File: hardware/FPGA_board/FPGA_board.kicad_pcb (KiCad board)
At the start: 6 copper layers, 50.9 x 24.8 mm, 142 parts, among them J1 USB_C_Receptacle_USB2.0, J2 Conn_01x6_Male, J3 USB_C_Receptacle_USB2.0, J4 MicroSd, J5 Conn_01x03, J6 JTAG, J7 Conn_02x15_Odd_Even, J8 Conn_02x15_Odd_Even, SW1 SW_Push, U1 RY1303 or EA3036, U10 NCP115-2.5, U3 ECP5U25, U4 MT41K64M16TW-107_J-TR, U6 XT25Q08DDTIGT, U8 TPS51206

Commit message: update PCB design files
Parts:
- added G***: LOGO, LOGO, B.Cu at (176.1, 92.9)
- added G***: LOGO, LOGO, B.Cu at (162.9, 93.3)

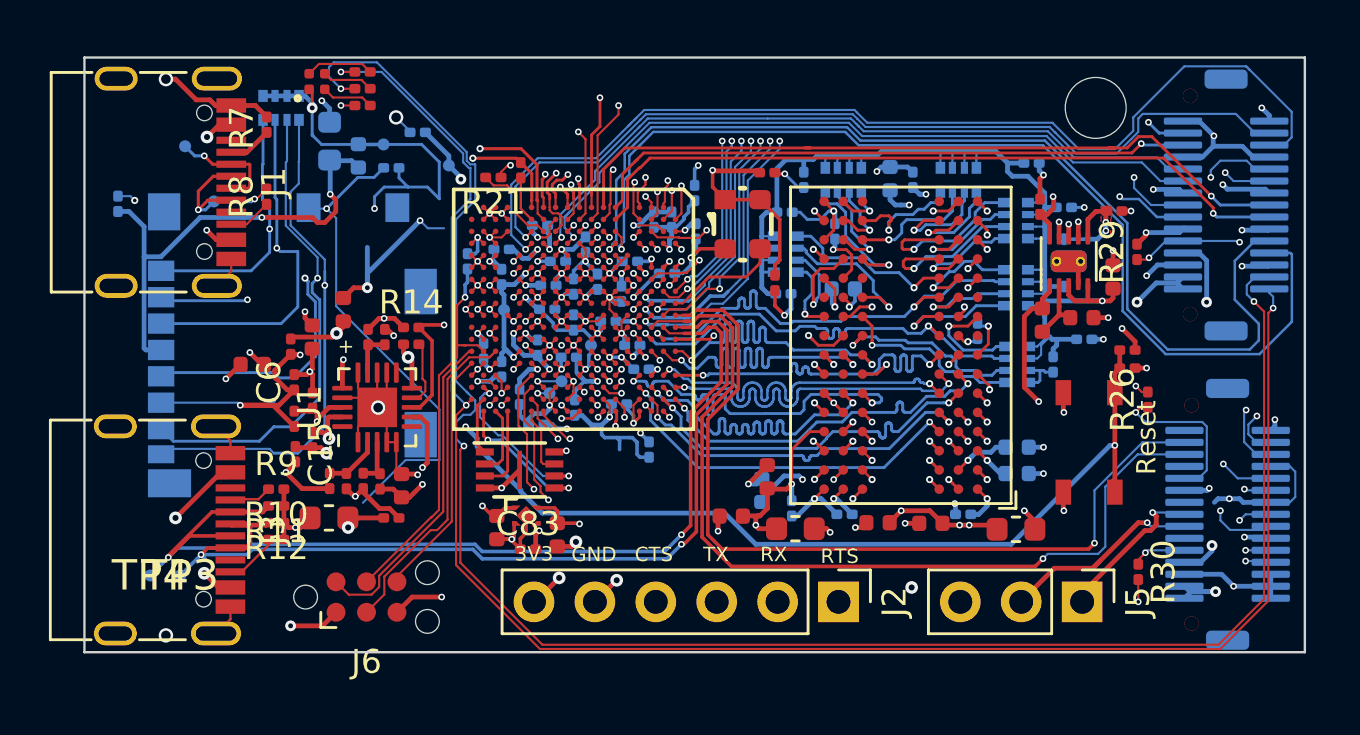
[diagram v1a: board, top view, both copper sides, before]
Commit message: update PCB design files
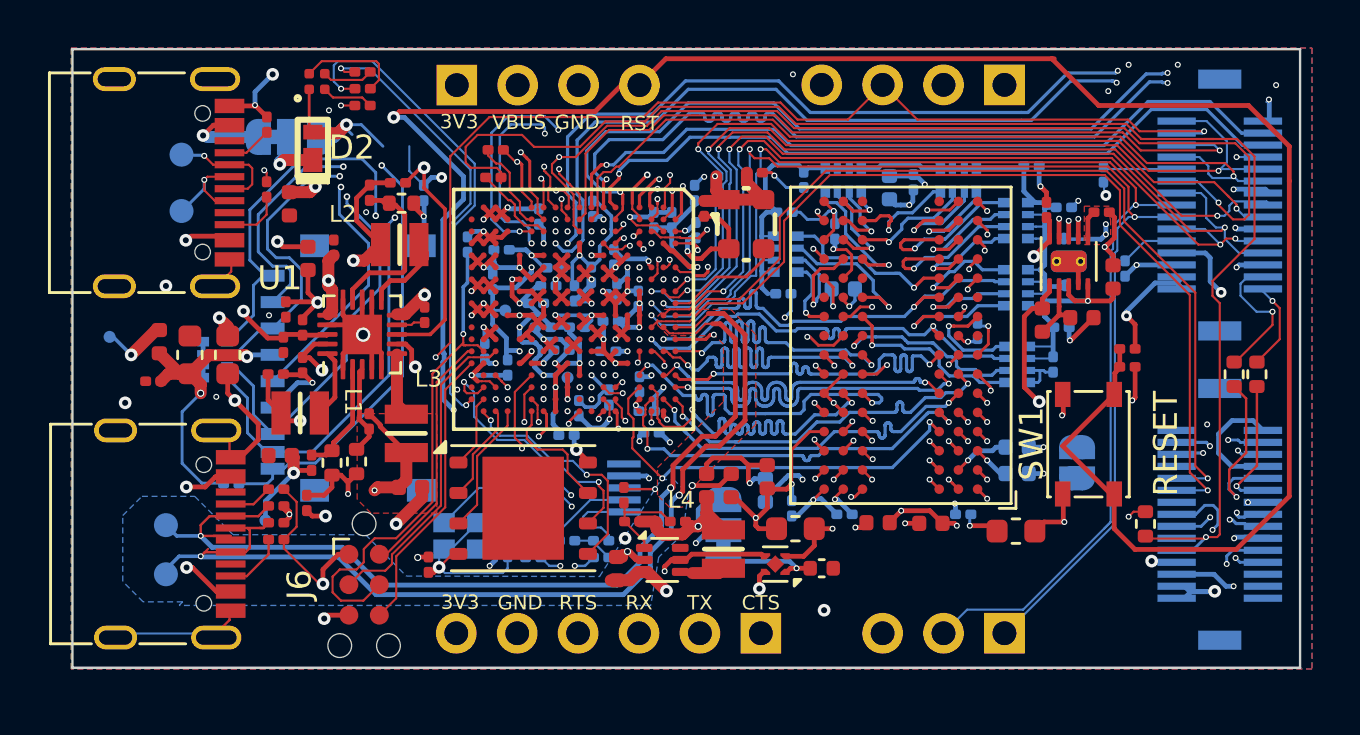
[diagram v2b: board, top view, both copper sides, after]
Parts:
- removed the G*** at (176.1, 92.9)
- removed the G*** at (162.9, 93.3)
- removed H4: MountingHole, MountingHole:MountingHole_2.1mm
- removed J1, J3: USB_C_Receptacle_USB2.0, Connector_USB:USB_C_Receptacle_G-Switch_GT-USB-7010ASV
- removed TP19, TP20: SMD_TP, gkl_misc:TestPoint_Pad_D0.5mm
- removed TP3, TP4: , 
- removed U10: NCP115-2.5, gkl_housings_son:X2SON_4_1.0x1.0mm
- added C13: 100pF, Capacitor_SMD:C_0201_0603Metric, F.Cu at (164.8, 109.8)
- added C28: 4.7uF, Capacitor_SMD:C_0402_1005Metric, F.Cu at (170.8, 111.7)
- added C29: 100nF, Capacitor_SMD:C_0201_0603Metric, B.Cu at (157.7, 110.9)
- added D2: D_Schottky, Library:U-DFN1608-2_L1.6-W0.8-RD, F.Cu at (149.5, 94.1)
- added G***: LOGO, LOGO, B.Cu at (171.0, 104.0)
- added G***: LOGO, LOGO, B.Cu at (182.6, 109.8)
- added J10: Conn_01x04, Connector_PinHeader_2.54mm:PinHeader_1x04_P2.54mm_Vertical, B.Cu at (155.5, 91.5)
- added J9: TF TF-018 1.5mm, Library:TF-SMD_TF-018, B.Cu at (149.7, 103.6)
- added JP1: SolderJumper_3_Bridged12, Jumper:SolderJumper-3_P1.3mm_Bridged12_RoundedPad1.0x1.5mm, B.Cu at (148.5, 93.7)
- added JP2: SolderJumper_3_Bridged12, Jumper:SolderJumper-3_P1.3mm_Bridged12_RoundedPad1.0x1.5mm, B.Cu at (166.7, 110.1)
- added JP3: SolderJumper_2_Open, Jumper:SolderJumper-2_P1.3mm_Open_RoundedPad1.0x1.5mm, B.Cu at (181.4, 107.3)
- added L1: 2.2uH, Library:Murata_DFE201612P-2R2M=P2, F.Cu at (149.0, 105.2)
- added L2: 2.2uH, Library:Murata_DFE201612P-2R2M=P2, F.Cu at (153.2, 98.2)
- added L3: 2.2uH, Library:Murata_DFE201612P-2R2M=P2, F.Cu at (153.4, 106.1)
- added L4: 2.2uH, Library:Murata_DFE201612P-2R2M=P2, F.Cu at (166.7, 110.9)
- added R31: 22, Resistor_SMD:R_0402_1005Metric, F.Cu at (188.9, 103.6)
- added R32: 22, Resistor_SMD:R_0402_1005Metric, F.Cu at (187.9, 103.6)
- added R33: 15k, Resistor_SMD:R_0201_0603Metric, F.Cu at (162.8, 109.8)
- added R34: 4.7k, Resistor_SMD:R_0201_0603Metric, F.Cu at (162.5, 108.7)
- added R35: 15, Resistor_SMD:R_0201_0603Metric, B.Cu at (161.6, 110.5)
- added R36: 15, Resistor_SMD:R_0201_0603Metric, B.Cu at (158.7, 110.5)
- added R37: 75, Resistor_SMD:R_0201_0603Metric, B.Cu at (160.1, 110.5)
- added R38: 15, Resistor_SMD:R_0201_0603Metric, B.Cu at (161.6, 111.2)
- added R39: 15, Resistor_SMD:R_0201_0603Metric, B.Cu at (158.7, 111.2)
- added TP1: SMD_TP, TestPoint:TestPoint_Pad_D1.0mm, B.Cu at (143.4, 112.0)
- added TP2: SMD_TP, TestPoint:TestPoint_Pad_D1.0mm, B.Cu at (143.4, 109.9)
- added U2: TLV62569APDRL, Package_TO_SOT_SMD:SOT-563, F.Cu at (164.1, 111.3)
- added U5: Si5351A-B-GT, Package_SO:MSOP-10_3x3mm_P0.5mm, B.Cu at (160.3, 108.3)
- added U7: NCP115AMX250TCG, Package_DFN_QFN:OnSemi_XDFN4-1EP_1.0x1.0mm_EP0.52x0.52mm, F.Cu at (168.8, 111.5)
- added USBD1: USB_C_Receptacle_USB2.0, Connector_USB:USB_C_Receptacle_G-Switch_GT-USB-7010ASV, F.Cu at (142.3, 95.6)
- added USBH1: USB_C_Receptacle_USB2.0, Connector_USB:USB_C_Receptacle_G-Switch_GT-USB-7010ASV, F.Cu at (142.4, 110.3)
- added Y1: 27MHz, Crystal:Crystal_SMD_2016-4Pin_2.0x1.6mm, B.Cu at (155.7, 110.3)
- C70, C71, FB1: moved to F.Cu
- J2, J5, R26, R30: moved to B.Cu
- J4: value MicroSd -> Conn_01x04_Male; footprint Connector_Card:microSD_HC_Molex_104031-0811 -> Connector_PinHeader_2.54mm:PinHeader_1x04_P2.54mm_Vertical
- J7, J8: footprint gkl_conn:DF12(3.0)-30DP-0.5V(86) -> Library:DF12NB3030DP05V51
- R10, R9: value 51K -> 12K
- R15: value 120K -> 120K 1%; footprint Resistor_SMD:R_0201_0603Metric -> Resistor_SMD:R_0402_1005Metric
- R16: value 82K -> 82K 1%; footprint Resistor_SMD:R_0201_0603Metric -> Resistor_SMD:R_0402_1005Metric
- R17, R18, R5: value 100k -> 100k 1%
- R2: value 22K -> 22K 1%; footprint Resistor_SMD:R_0201_0603Metric -> Resistor_SMD:R_0402_1005Metric
- R29: footprint Resistor_SMD:R_0201_0603Metric -> Resistor_SMD:R_0402_1005Metric
- SW1: footprint gkl_misc:PTS_810_SMT_Switch -> Button_Switch_SMD:SW_SPST_PTS810
- TP26, TP27: footprint gkl_misc:TestPoint_Pad_D0.5mm -> TestPoint:TestPoint_Pad_D1.0mm
- TP28, TP29, TP30, TP31, TP32, TP33: footprint gkl_misc:TestPoint_Pad_D0.5mm -> Library:TestPoint_Pad_D0.5mm
- U3: value ECP5U25 -> ECP5
- U6: value XT25Q08DDTIGT -> W25Q128JVPIQ; footprint gkl_housings_dfn:DFN-8-1EP_3x2mm_Pitch0.5mm -> Package_SON:WSON-8-1EP_6x5mm_P1.27mm_EP3.4x4.3mm
- moved J4 31.6 mm to (178.4, 91.5), turned to 90 degrees
- moved TP32 15.4 mm to (147.6, 109.7), turned to 180 degrees
- moved R28 14.8 mm to (146.1, 108.2), turned to 0 degrees
- moved TP29 14.0 mm to (141.1, 102.0), turned to 180 degrees
- moved R30 12.7 mm to (183.4, 99.2)
- moved FB1 11.4 mm to (143.1, 102.2)
- moved R29 11.4 mm to (184.2, 109.8)
- moved RN7 10.9 mm to (145.4, 103.0), turned to 180 degrees
- moved C71 10.6 mm to (144.4, 102.8)
- moved TP31 10.1 mm to (160.2, 103.8), turned to 180 degrees
- moved R26 9.58 mm to (182.5, 95.3), turned to -90 degrees
- moved C47 8.93 mm to (165.9, 108.2), turned to 90 degrees
- moved C3 8.01 mm to (146.0, 102.8), turned to 90 degrees
- moved C70 7.55 mm to (142.9, 103.9), turned to 0 degrees
- moved R14 6.06 mm to (153.1, 95.6)
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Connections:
- net USB_PULLUP renamed PULLUP_USB
- C11 pad 1: GND -> VTT
- C11 pad 2: VTT -> GND
- C14 pad 2: PUSB_VBUS -> VSYS
- C17 pad 1: GND -> P1.1V
- C17 pad 2: P1.1V -> GND
- C18 pad 1: GND -> P1.35V
- C18 pad 2: P1.35V -> GND
- C2 pad 2: PUSB_VBUS -> VSYS
- C3 pad 2: PUSB_VBUS -> VSYS
- C47 pad 1: P2.5V -> Net-(JP2-B)
- C5 pad 2: PUSB_VBUS -> VSYS
- C7 pad 1: GND -> P3.3V
- C7 pad 2: P3.3V -> GND
- C70 pad 2: Net-(J4-Pin_4) -> /sheetSDMMC/VDD_SD
- C71 pad 1: Net-(J4-Pin_4) -> /sheetSDMMC/VDD_SD
- FB1 pad 1: Net-(J4-Pin_4) -> /sheetSDMMC/VDD_SD
- J2 pad 1: IO_1 -> IO_MISO
- J2 pad 2: IO_0 -> IO_1
- J2 pad 3: IO_MISO -> IO_0
- J4 pad 1: SD0_DAT2 -> IO_10
- J4 pad 2: SD0_DAT3 -> IO_9
- J4 pad 3: SD0_CMD -> IO_SCK
- J4 pad 4: Net-(J4-Pin_4) -> IO_13
- J5 pad 1: IO_SDA -> IO_SCL
- J5 pad 2: IO_SCL -> IO_SDA
- J7 pad 1: GND -> IO_11
- J7 pad 10: AUX_1- -> IO_11
- J7 pad 11: AUX_4+ -> LED_B
- J7 pad 12: AUX_1+ -> IO_12
- J7 pad 13: GND -> IO_6
- J7 pad 15: AUX_5- -> IO_SDA
- J7 pad 16: AUX_2- -> IO_9
- J7 pad 17: AUX_5+ -> IO_SCL
- J7 pad 18: AUX_2+ -> IO_10
- J7 pad 19: GND -> IO_5
- J7 pad 21: HPD/ID -> Net-(J7-Pin_21)
- J7 pad 22: AUX_6+ -> IO_5
- J7 pad 24: AUX_6- -> IO_6
- J7 pad 28: LED_G -> Net-(J7-Pin_28)
- J7 pad 3: AUX_3- -> IO_SCK
- J7 pad 30: LED_R -> Net-(J7-Pin_30)
- J7 pad 4: AUX_0- -> AUX_3-
- J7 pad 5: AUX_3+ -> IO_13
- J7 pad 6: AUX_0+ -> AUX_3+
- J7 pad 7: GND -> IO_12
- J7 pad 9: AUX_4- -> Net-(J7-Pin_9)
- J7 pad MP: (no net) -> GND
- J8 pad 10: IO_11 -> AUX_1-
- J8 pad 11: LED_B -> SPI_1
- J8 pad 12: IO_12 -> AUX_1+
- J8 pad 15: IO_SDA -> AUX_5-
- J8 pad 16: IO_9 -> AUX_2-
- J8 pad 17: IO_SCL -> AUX_5+
- J8 pad 18: IO_10 -> AUX_2+
- J8 pad 21: Net-(J8-Pin_21) -> HPD/ID
- J8 pad 22: IO_5 -> AUX_6+
- J8 pad 24: IO_6 -> AUX_6-
- J8 pad 3: SPI_0 -> AUX_4-
- J8 pad 4: IO_SCK -> AUX_0-
- J8 pad 5: SPI_1 -> AUX_4+
- J8 pad 6: IO_13 -> AUX_0+
- J8 pad 9: Net-(J8-Pin_9) -> SPI_0
- J8 pad MP: (no net) -> GND
- R10 pad 1: Net-(J3-CC2) -> P3.3V
- R10 pad 2: GND -> Net-(USBH1-CC2)
- R22 pad 1: LED_R -> LED_G
- R23 pad 1: LED_G -> LED_R
- R26 pad 1: Net-(J8-Pin_9) -> Net-(J7-Pin_9)
- R28 pad 1: P3.3V -> /sheetSDMMC/VDD_SD
- R30 pad 1: Net-(J8-Pin_21) -> Net-(J7-Pin_21)
- R9 pad 1: Net-(J3-CC1) -> P3.3V
- R9 pad 2: GND -> Net-(USBH1-CC1)
- RN7 pad 1: SD0_DAT1 -> SD0_DAT2
- RN7 pad 2: SD0_DAT0 -> SD0_CMD
- RN7 pad 3: SD0_CMD -> SD0_DAT0
- RN7 pad 4: SD0_DAT2 -> SD0_DAT1
- RN7 pad 5: P3.3V -> /sheetSDMMC/VDD_SD
- RN7 pad 6: P3.3V -> /sheetSDMMC/VDD_SD
- RN7 pad 7: P3.3V -> /sheetSDMMC/VDD_SD
- RN7 pad 8: P3.3V -> /sheetSDMMC/VDD_SD
- U1 pad 16: PUSB_VBUS -> VSYS
- U1 pad 19: PUSB_VBUS -> VSYS
- U1 pad 7: PUSB_VBUS -> VSYS
- U4 pad G8: (no net) -> GND
- U4 pad J1: (no net) -> unconnected-(U4-PadJ1)
- U4 pad J9: (no net) -> unconnected-(U4-PadJ9)
- U4 pad L1: (no net) -> unconnected-(U4-PadL1)
- U4 pad L9: (no net) -> unconnected-(U4-PadL9)
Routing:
- net P3.3V: track 174.3 -> 241.5 mm, vias 22 -> 21
- net LED_G: track 80.7 -> 22.8 mm, vias 4 -> 3
- net LED_R: track 74.8 -> 18.7 mm, vias 3 -> 2
- net FPGA_RESET: track 41.1 -> 90.9 mm
- net VSYS: track 0.00 -> 44.7 mm, vias 0 -> 6
- net /sheetHyperRAM/RAM_VDD: track 18.1 -> 60.0 mm, vias 12 -> 11
- net IO_SDA: track 44.1 -> 73.9 mm, vias 3 -> 4
- net AUX_2+: track 30.2 -> 57.3 mm, vias 1 -> 3
- net IO_SCL: track 47.5 -> 73.6 mm, vias 3 -> 4
- net AUX_4+: track 30.6 -> 55.5 mm, vias 1 -> 3
- net AUX_4-: track 30.1 -> 54.9 mm, vias 1 -> 3
- net AUX_2-: track 31.7 -> 55.4 mm, vias 1 -> 3
- net /sheetPower/PGOOD_P1.1V: track 16.5 -> 38.3 mm, vias 2 -> 3
- net /sheetHyperRAM/RAM_VDDQ: track 15.6 -> 36.4 mm
- net AUX_1-: track 34.4 -> 54.9 mm
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- added copper zone on In2.Cu, net (none)
- added copper zone on B.Cu, net GND
- added copper zone on F.Cu, net GND
- added copper zone on F.Cu, net P1.35V
- added copper zone on In1.Cu, net P1.35V
- added copper zone on In2.Cu, net P2.5V
- added copper zone on In2.Cu, net P3.3V
- added copper zone on In1.Cu, net PUSB_VBUS
- added copper zone on In3.Cu, net VSYS
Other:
- board size 50.9 x 24.8 mm -> 51.2 x 25.8 mm
- board text added: "0.275/.15 via handles 1.6A .53/.25 via handles 2.2A .5 track (external) handles 1.4A .2 track (external) handles .73A internal tracks: 5x"
- board text added: "90ohm JLC06161H-3313A coplanar -trace spacing/clearance: .2032mm width: .1554mm"
- board text added: "Avaota-A1 design BGA pad: 0.2285 track: 0.076 clearance: 0.09775 via-in-pad: 0.4/0.3 ovals: 0.2-0.305 (replacing .25) Soldermask: matches BGA pad"
- board text added: "DEV"
- board text added: "FPGA board"
- board text added: "G"
- board text added: "HOST"
- board text added: "Hole to pad distance should be made greater (.18 to .22-.25)"
- board text added: "PCB3D_BR_FPGA_board"
- board text added: "PCB3D_TL_FPGA_board"
- board text added: "RESET"
- board text added: "The design is according to: https://jlcpcb.com/help/article/243-BGA-Design-Guidelines---PCB-Layout-Recommendations-for-BGA-packages That means: 0.25mm BGA pad and Via-In-Pad outer diameter 0.15mm Via holes 0.09mm Minimum for normal tracks 0.076mm Tracks passing between BGA pads (infrequent)"
- board text added: "VBUS"
- board text removed: "+"
- board text removed: "Micro SD"
- board text removed: "Reset"
